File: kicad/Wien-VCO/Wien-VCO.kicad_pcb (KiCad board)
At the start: 2 copper layers, 61.1 x 45.8 mm, 30 parts, among them J1 J113, U1 MAX4104

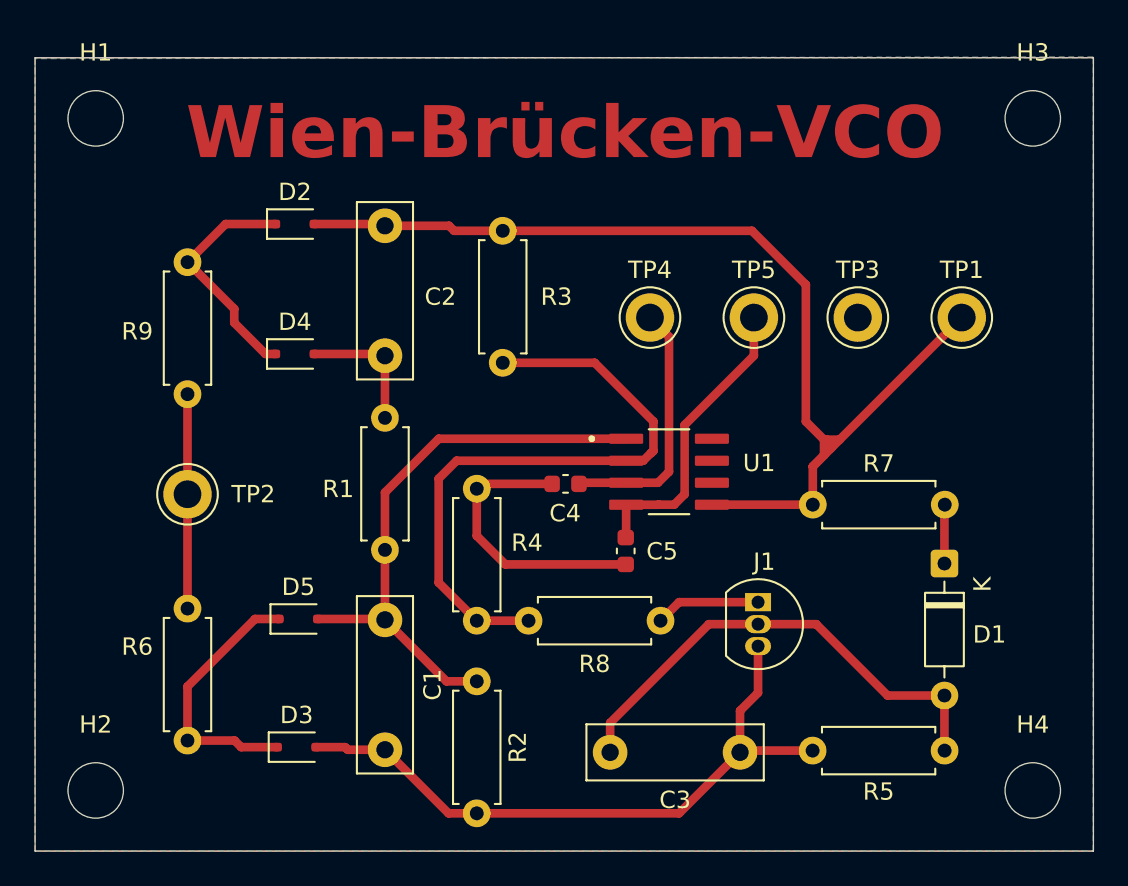
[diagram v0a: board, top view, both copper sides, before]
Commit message: Layout finalisiert
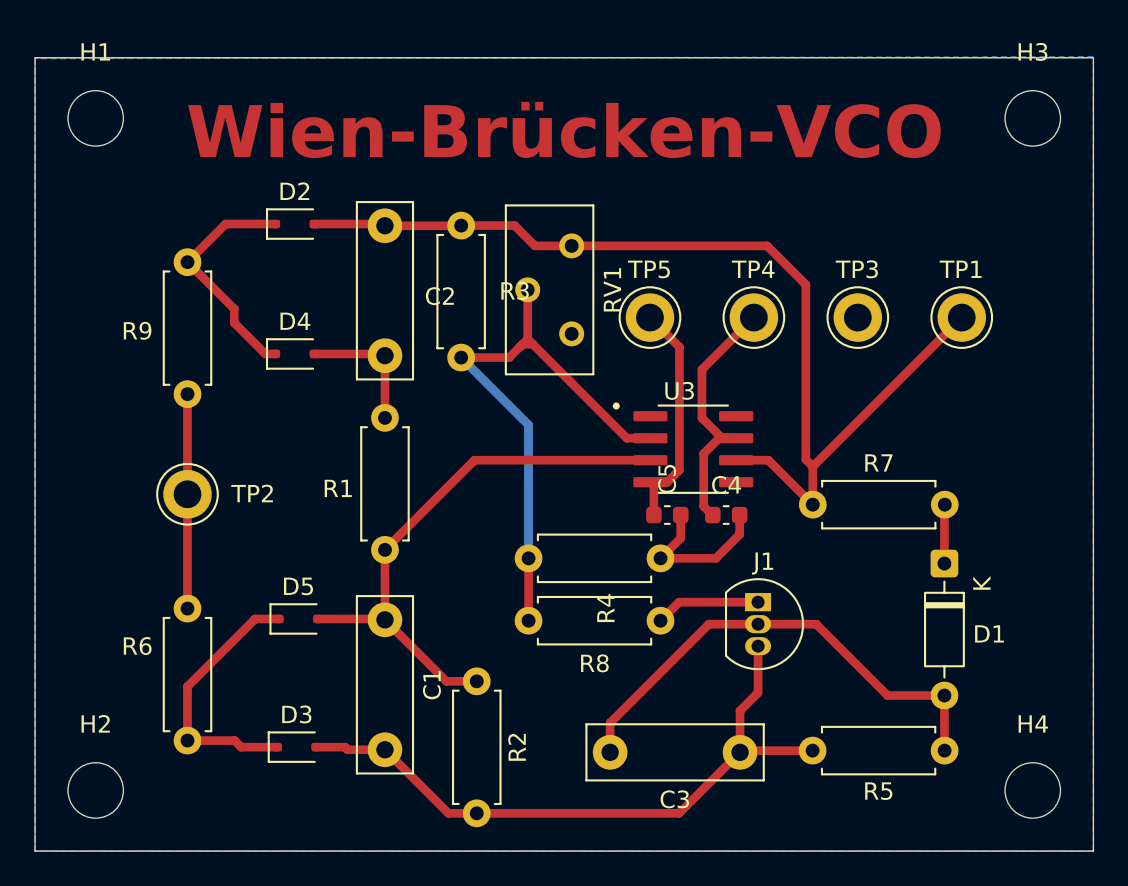
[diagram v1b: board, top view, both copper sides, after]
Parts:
- removed U1: MAX4104, Library:SOIC8-Adapter
- added RV1: R_Potentiometer, Potentiometer_THT:Potentiometer_Bourns_3296Y_Vertical, F.Cu at (168.5, 82.9)
- added U3: MAX4104ESA_, Library:SOIC127P600X175-8N_neu, F.Cu at (175.5, 89.6)
- moved C4 9.45 mm to (177.4, 93.4), turned to 180 degrees
- moved TP4 6.00 mm to (179.0, 82.0)
- moved TP5 6.00 mm to (173.0, 82.0)
- moved R4 4.68 mm to (166.0, 95.9), turned to 0 degrees
- moved C5 3.17 mm to (174.0, 93.4), turned to 180 degrees
- moved R3 2.42 mm to (162.1, 84.3)
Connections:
- net /Va renamed Va
- net /Ve renamed Ve
- net Net-(D5-A) renamed V2
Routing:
- net 0: track 54.8 -> 47.6 mm
- net VCC-: track 17.4 -> 13.5 mm
- net Ve: track 37.0 -> 34.2 mm
- net Va: track 62.7 -> 60.1 mm
- net V2: track 33.4 -> 32.3 mm
- net VCC+: track 14.8 -> 15.5 mm
